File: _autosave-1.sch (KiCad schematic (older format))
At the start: 56 parts, among them J1 ValveOUT, J10 PD6, J2 220V_IN, J3 MotorOUT, J4 PumpOUT, J5 ISCP, J6 ButtonOUT, J7 SwitchOUT, J8 FloatOUT, J9 LedOUT, Q1 BT136, Q2 BT136, Q3 BT136, SW1 SW_Push, U1 ATmega8A-AU, U2 MOC3023M, U3 MOC3023M, U4 MOC3023M, Y1 16MHz

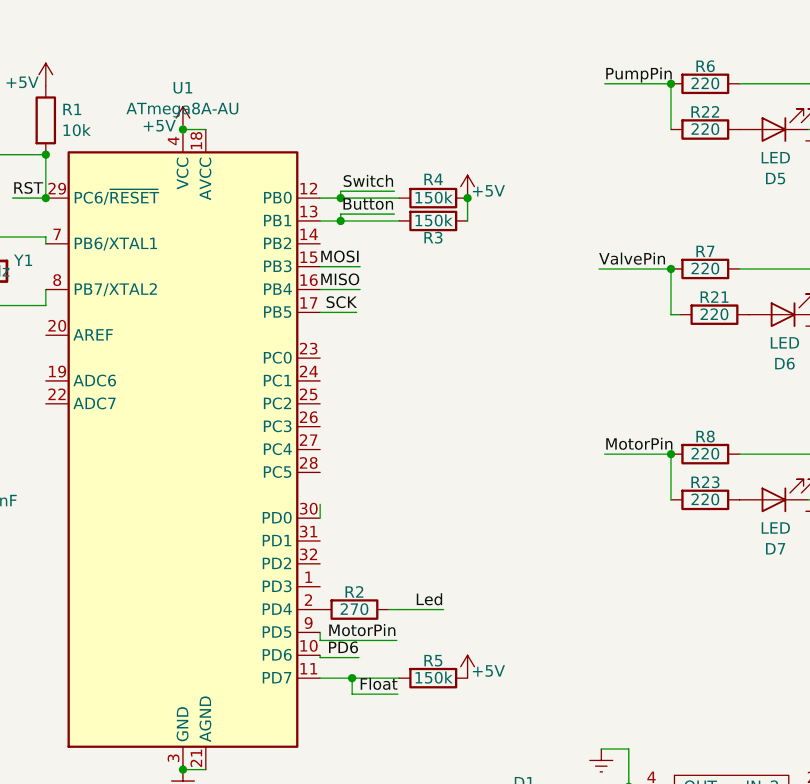
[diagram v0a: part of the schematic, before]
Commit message: 5.0
Плата готова
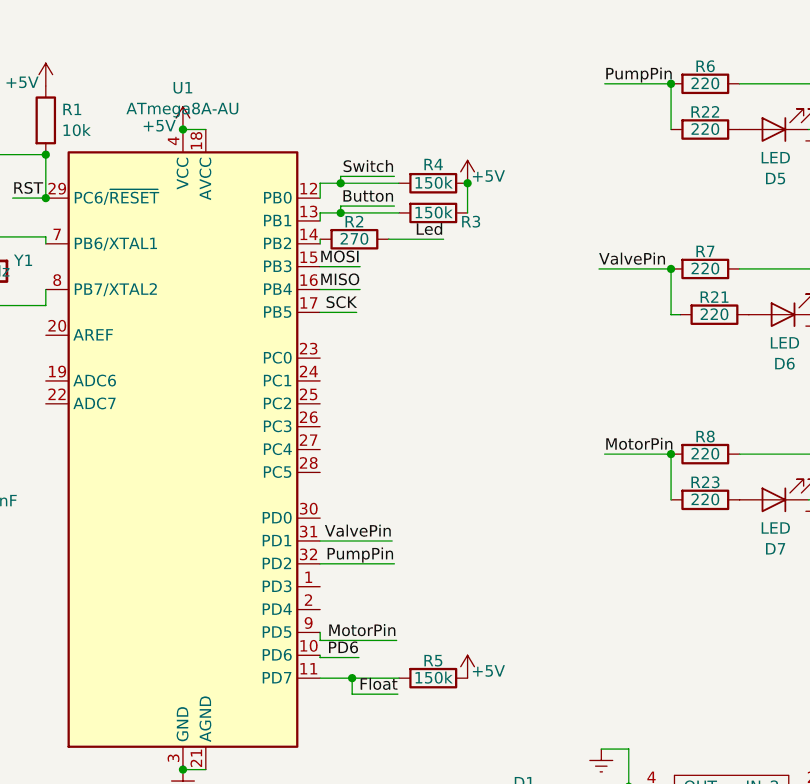
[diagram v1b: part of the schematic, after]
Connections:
- net PumpPin: now also U1.32 (PD2)
- net ValvePin: now also U1.31 (PD1)
- net at U1.14 (PB2): now also R2.2
- net at U1.2 (PD4): no longer R2.2
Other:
- moved on the sheet: R2, R3, R4
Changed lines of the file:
@@
 	6915 4775 7215 4775
-$Comp
-L Device:R R3
-U 1 1 5DE7B4F3
-P 4190 2220
-F 0 "R3" V 4265 2220 50  0000 C CNN
-F 1 "150k" V 4190 2220 50  0000 C CNN
-F 2 "Resistors_SMD:R_1206" V 4120 2220 50  0001 C CNN
-F 3 "~" H 4190 2220 50  0001 C CNN
-	1    4190 2220
-	0    1    1    0
-$EndComp
 $Comp
 L Device:R R5
@@
 	0    1    1    0
 $EndComp
-Text Label 4020 2190 2    50   ~ 0
+Text Label 4020 2155 2    50   ~ 0
 Button
 $Comp
@@
 Wire Wire Line
 	8520 3115 8295 3115
-Wire Wire Line
-	3695 3460 3695 3520
-Wire Wire Line
-	3695 2220 3785 2220
-Wire Wire Line
-	3785 2220 3785 2190
-Wire Wire Line
-	3785 2190 4020 2190
-Connection ~ 3785 2220
-Wire Wire Line
-	3785 2220 4040 2220
 $Comp
 L power:Earth #PWR0112
@@
 L Device:R R2
 U 1 1 5DFECCE6
-P 3845 3920
-F 0 "R2" V 3770 3920 50  0000 C CNN
-F 1 "270" V 3845 3920 50  0000 C CNN
-F 2 "Resistors_SMD:R_1206" V 3775 3920 50  0001 C CNN
-F 3 "~" H 3845 3920 50  0001 C CNN
-	1    3845 3920
-	0    1    1    0
-$EndComp
-Wire Wire Line
-	3995 3920 4235 3920
-Text Label 4235 3920 2    50   ~ 0
+P 3845 2300
+F 0 "R2" V 3770 2300 50  0000 C CNN
+F 1 "270" V 3845 2300 50  0000 C CNN
+F 2 "Resistors_SMD:R_1206" V 3775 2300 50  0001 C CNN
+F 3 "~" H 3845 2300 50  0001 C CNN
+	1    3845 2300
+	0    1    1    0
+$EndComp
+Wire Wire Line
+	3995 2300 4235 2300
+Text Label 4235 2300 2    50   ~ 0
 Led
 $Comp
@@
 Wire Wire Line
 	8455 3645 8325 3645
-Text Label 4940 3240 0    50   ~ 0
-MotorPin
 Text Label 4940 1620 0    50   ~ 0
 PumpPin
@@
 Text Label 4915 2430 0    50   ~ 0
 ValvePin
-Wire Wire Line
-	5230 3240 4940 3240
-Connection ~ 5230 3240
 Text Label 4030 4055 2    50   ~ 0
 MotorPin
@@
 Connection ~ 5230 1620
 Wire Wire Line
-	3785 2120 3695 2120
-Wire Wire Line
-	3785 2090 4020 2090
-Wire Wire Line
-	3785 2120 3785 2090
-Wire Wire Line
-	4040 2120 3785 2120
+	3785 2055 3695 2055
+Wire Wire Line
+	3785 2025 4020 2025
+Wire Wire Line
+	3785 2055 3785 2025
+Wire Wire Line
+	4040 2055 3785 2055
 $Comp
 L Device:R R4
 U 1 1 5DF5A9F9
-P 4190 2120
-F 0 "R4" V 4110 2120 50  0000 C CNN
-F 1 "150k" V 4190 2120 50  0000 C CNN
-F 2 "Resistors_SMD:R_1206" V 4120 2120 50  0001 C CNN
-F 3 "~" H 4190 2120 50  0001 C CNN
-	1    4190 2120
-	0    1    1    0
-$EndComp
-Text Label 4020 2090 2    50   ~ 0
+P 4190 2055
+F 0 "R4" V 4110 2055 50  0000 C CNN
+F 1 "150k" V 4190 2055 50  0000 C CNN
+F 2 "Resistors_SMD:R_1206" V 4120 2055 50  0001 C CNN
+F 3 "~" H 4190 2055 50  0001 C CNN
+	1    4190 2055
+	0    1    1    0
+$EndComp
+Text Label 4020 2025 2    50   ~ 0
 Switch
 $Comp
-L power:+5V #PWR?
+L power:+5V #PWR0116
 U 1 1 5DF9338B
-P 4340 2120
-F 0 "#PWR?" H 4340 1970 50  0001 C CNN
-F 1 "+5V" H 4430 2150 50  0000 C CNN
-F 2 "" H 4340 2120 50  0001 C CNN
-F 3 "" H 4340 2120 50  0001 C CNN
-	1    4340 2120
+P 4340 2055
+F 0 "#PWR0116" H 4340 1905 50  0001 C CNN
+F 1 "+5V" H 4430 2085 50  0000 C CNN
+F 2 "" H 4340 2055 50  0001 C CNN
+F 3 "" H 4340 2055 50  0001 C CNN
+	1    4340 2055
 	1    0    0    -1
 $EndComp
@@
 	5230 2430 4915 2430
 Connection ~ 5230 2430
-Connection ~ 3785 2120
-Wire Wire Line
-	4340 2220 4340 2120
-Connection ~ 4340 2120
+Connection ~ 3785 2055
+Connection ~ 4340 2055
+Wire Wire Line
+	3695 2120 3695 2055
+Wire Wire Line
+	3785 2155 4020 2155
+Wire Wire Line
+	3785 2185 3785 2155
+$Comp
+L Device:R R3
+U 1 1 5DE7B4F3
+P 4190 2185
+F 0 "R3" V 4230 2350 50  0000 C CNN
+F 1 "150k" V 4190 2185 50  0000 C CNN
+F 2 "Resistors_SMD:R_1206" V 4120 2185 50  0001 C CNN
+F 3 "~" H 4190 2185 50  0001 C CNN
+	1    4190 2185
+	0    1    1    0
+$EndComp
+Wire Wire Line
+	4340 2055 4340 2185
+Wire Wire Line
+	4040 2185 3785 2185
+Wire Wire Line
+	3695 2185 3695 2220
+Connection ~ 3785 2185
+Wire Wire Line
+	3785 2185 3695 2185
+Wire Wire Line
+	3695 2300 3695 2320
+Connection ~ 5230 3240
+Wire Wire Line
+	5230 3240 4940 3240
+Text Label 4940 3240 0    50   ~ 0
+MotorPin
+Text Label 4010 3620 2    50   ~ 0
+ValvePin
+Wire Wire Line
+	3695 3620 4010 3620
+Text Label 4020 3720 2    50   ~ 0
+PumpPin
+Wire Wire Line
+	3695 3720 4020 3720
 $EndSCHEMATC
